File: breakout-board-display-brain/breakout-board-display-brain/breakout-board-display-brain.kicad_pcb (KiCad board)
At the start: 2 copper layers, 41 x 68.7 mm, 6 parts, among them J1 Conn_01x19_Socket, J2 Conn_01x19_Socket, J3 Conn_01x02_Socket, J4 Conn_01x04_Socket, J5 Conn_01x04_Socket, SW1 RotaryEncoder_Switch

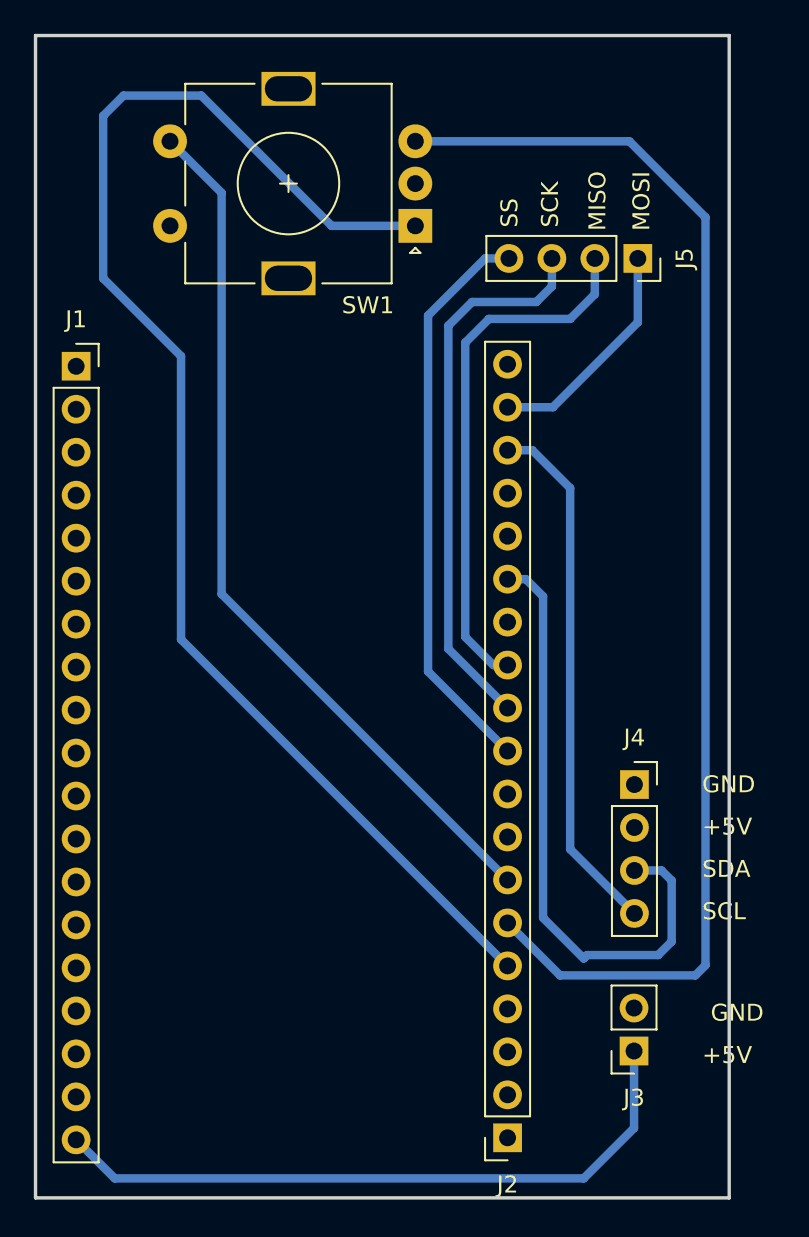
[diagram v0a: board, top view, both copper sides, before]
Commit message: ...
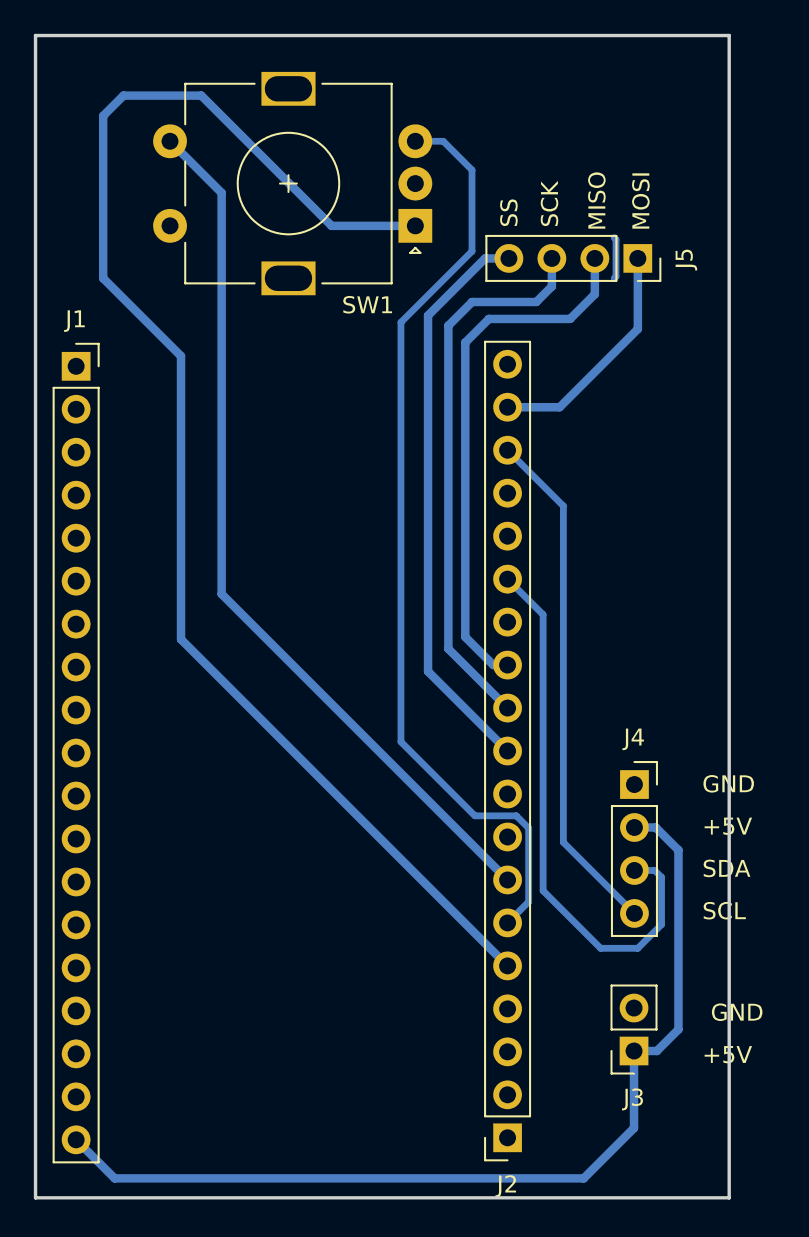
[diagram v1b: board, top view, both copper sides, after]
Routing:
- net /IO0: track 76.4 -> 55.4 mm
- net +5V: track 39.7 -> 56.6 mm
- net /IO21_SDA: track 36.6 -> 32.8 mm
- net GND: track 0.00 -> 3.07 mm
- net /IO22_SCL: track 31.3 -> 30.5 mm
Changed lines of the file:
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@@
     (effects (font (size 1 1) (thickness 0.15)) (justify left bottom))
   )
+  (segment (start 160.8 70.4) (end 160.91 70.51) (width 0.4) (layer "B.Cu") (net 1))
+  (segment (start 154.5 93.12) (end 154.5 93.7) (width 0.4) (layer "B.Cu") (net 1))
+  (segment (start 160.91 72.69) (end 160.8 72.8) (width 0.4) (layer "B.Cu") (net 1))
+  (segment (start 160.91 70.51) (end 160.91 72.69) (width 0.4) (layer "B.Cu") (net 1))
   (segment (start 159 126) (end 131.28 126) (width 0.5) (layer "B.Cu") (net 19))
   (segment (start 161.975 123.025) (end 161.975 118.47) (width 0.5) (layer "B.Cu") (net 19))
+  (segment (start 163.33 118.47) (end 161.975 118.47) (width 0.5) (layer "B.Cu") (net 19))
+  (segment (start 164.6 106.6) (end 164.6 117.2) (width 0.5) (layer "B.Cu") (net 19))
+  (segment (start 162 105.26) (end 163.26 105.26) (width 0.5) (layer "B.Cu") (net 19))
   (segment (start 159 126) (end 161.975 123.025) (width 0.5) (layer "B.Cu") (net 19))
+  (segment (start 163.26 105.26) (end 164.6 106.6) (width 0.5) (layer "B.Cu") (net 19))
   (segment (start 131.28 126) (end 129 123.72) (width 0.5) (layer "B.Cu") (net 19))
+  (segment (start 164.6 117.2) (end 163.33 118.47) (width 0.5) (layer "B.Cu") (net 19))
   (segment (start 135.2 77.4) (end 135.2 94.14) (width 0.5) (layer "B.Cu") (net 24))
   (segment (start 130.6 63.2) (end 130.6 72.8) (width 0.5) (layer "B.Cu") (net 24))
@@
   (segment (start 131.8 62) (end 130.6 63.2) (width 0.5) (layer "B.Cu") (net 24))
   (segment (start 136.4 62) (end 131.8 62) (width 0.5) (layer "B.Cu") (net 24))
-  (segment (start 149.05 64.7) (end 161.7 64.7) (width 0.5) (layer "B.Cu") (net 25))
-  (segment (start 165.6 114) (end 157.6 114) (width 0.5) (layer "B.Cu") (net 25))
-  (segment (start 161.7 64.7) (end 166.2 69.2) (width 0.5) (layer "B.Cu") (net 25))
-  (segment (start 166.2 113.4) (end 165.6 114) (width 0.5) (layer "B.Cu") (net 25))
-  (segment (start 157.6 114) (end 154.5 110.9) (width 0.5) (layer "B.Cu") (net 25))
-  (segment (start 166.2 69.2) (end 166.2 113.4) (width 0.5) (layer "B.Cu") (net 25))
+  (segment (start 152.4 66.4) (end 152.4 71.2) (width 0.4) (layer "B.Cu") (net 25))
+  (segment (start 150.7 64.7) (end 152.4 66.4) (width 0.4) (layer "B.Cu") (net 25))
+  (segment (start 155.75 105.302233) (end 155.75 109.65) (width 0.4) (layer "B.Cu") (net 25))
+  (segment (start 155.75 109.65) (end 154.5 110.9) (width 0.4) (layer "B.Cu") (net 25))
+  (segment (start 148.2 100.2) (end 152.57 104.57) (width 0.4) (layer "B.Cu") (net 25))
+  (segment (start 155.017767 104.57) (end 155.75 105.302233) (width 0.4) (layer "B.Cu") (net 25))
+  (segment (start 149.05 64.7) (end 150.7 64.7) (width 0.4) (layer "B.Cu") (net 25))
+  (segment (start 148.2 75.4) (end 148.2 100.2) (width 0.4) (layer "B.Cu") (net 25))
+  (segment (start 152.57 104.57) (end 155.017767 104.57) (width 0.4) (layer "B.Cu") (net 25))
+  (segment (start 152.4 71.2) (end 148.2 75.4) (width 0.4) (layer "B.Cu") (net 25))
   (segment (start 137.6 91.46) (end 154.5 108.36) (width 0.5) (layer "B.Cu") (net 26))
   (segment (start 134.55 64.7) (end 137.6 67.75) (width 0.5) (layer "B.Cu") (net 26))
@@
   (segment (start 159.66 73.74) (end 158.2 75.2) (width 0.5) (layer "B.Cu") (net 31))
   (segment (start 159.66 71.625) (end 159.66 73.74) (width 0.5) (layer "B.Cu") (net 31))
-  (segment (start 163.6 107.8) (end 164.2 108.4) (width 0.5) (layer "B.Cu") (net 32))
-  (segment (start 159 113) (end 156.6 110.6) (width 0.5) (layer "B.Cu") (net 32))
-  (segment (start 156.6 110.6) (end 156.6 91.6) (width 0.5) (layer "B.Cu") (net 32))
-  (segment (start 155.58 90.58) (end 154.5 90.58) (width 0.5) (layer "B.Cu") (net 32))
-  (segment (start 156.6 91.6) (end 155.58 90.58) (width 0.5) (layer "B.Cu") (net 32))
-  (segment (start 162 107.8) (end 163.6 107.8) (width 0.5) (layer "B.Cu") (net 32))
-  (segment (start 164.2 112) (end 163.4 112.8) (width 0.5) (layer "B.Cu") (net 32))
-  (segment (start 159.2 112.8) (end 159 113) (width 0.5) (layer "B.Cu") (net 32))
-  (segment (start 163.4 112.8) (end 159.2 112.8) (width 0.5) (layer "B.Cu") (net 32))
-  (segment (start 164.2 108.4) (end 164.2 112) (width 0.5) (layer "B.Cu") (net 32))
-  (segment (start 158.2 106.54) (end 162 110.34) (width 0.5) (layer "B.Cu") (net 35))
-  (segment (start 155.96 82.96) (end 158.2 85.2) (width 0.5) (layer "B.Cu") (net 35))
-  (segment (start 154.5 82.96) (end 155.96 82.96) (width 0.5) (layer "B.Cu") (net 35))
-  (segment (start 158.2 85.2) (end 158.2 106.54) (width 0.5) (layer "B.Cu") (net 35))
-  (segment (start 157.18 80.42) (end 162.2 75.4) (width 0.5) (layer "B.Cu") (net 36))
-  (segment (start 154.5 80.42) (end 157.18 80.42) (width 0.5) (layer "B.Cu") (net 36))
-  (segment (start 162.2 75.4) (end 162.2 71.625) (width 0.5) (layer "B.Cu") (net 36))
+  (segment (start 156.6 109) (end 160 112.4) (width 0.4) (layer "B.Cu") (net 32))
+  (segment (start 163.6 111) (end 163.6 108.2) (width 0.4) (layer "B.Cu") (net 32))
+  (segment (start 160 112.4) (end 162.2 112.4) (width 0.4) (layer "B.Cu") (net 32))
+  (segment (start 156.6 92.68) (end 156.6 109) (width 0.4) (layer "B.Cu") (net 32))
+  (segment (start 163.2 107.8) (end 162 107.8) (width 0.4) (layer "B.Cu") (net 32))
+  (segment (start 163.6 108.2) (end 163.2 107.8) (width 0.4) (layer "B.Cu") (net 32))
+  (segment (start 154.5 90.58) (end 156.6 92.68) (width 0.4) (layer "B.Cu") (net 32))
+  (segment (start 162.2 112.4) (end 163.6 111) (width 0.4) (layer "B.Cu") (net 32))
+  (segment (start 162 110.34) (end 157.8 106.14) (width 0.4) (layer "B.Cu") (net 35))
+  (segment (start 157.8 106.14) (end 157.8 86.26) (width 0.4) (layer "B.Cu") (net 35))
+  (segment (start 157.8 86.26) (end 154.5 82.96) (width 0.4) (layer "B.Cu") (net 35))
+  (segment (start 157.58 80.42) (end 154.5 80.42) (width 0.5) (layer "B.Cu") (net 36))
+  (segment (start 162.2 75.8) (end 157.58 80.42) (width 0.5) (layer "B.Cu") (net 36))
+  (segment (start 162.2 71.625) (end 162.2 75.8) (width 0.5) (layer "B.Cu") (net 36))
   (zone (net 1) (net_name "GND") (layer "B.Cu") (hatch edge 0.5)
     (connect_pads (clearance 0.508))
